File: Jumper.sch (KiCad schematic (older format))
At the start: 4 parts, among them J6 Conn_Coaxial, J7 Conn_Coaxial

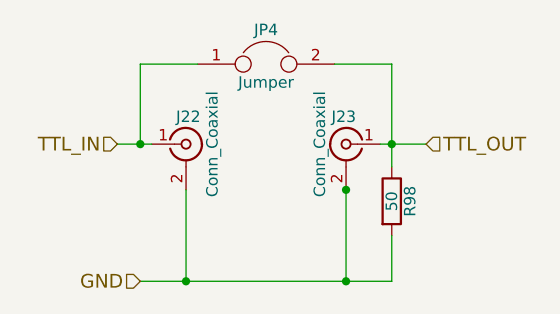
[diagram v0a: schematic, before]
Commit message: Version 1
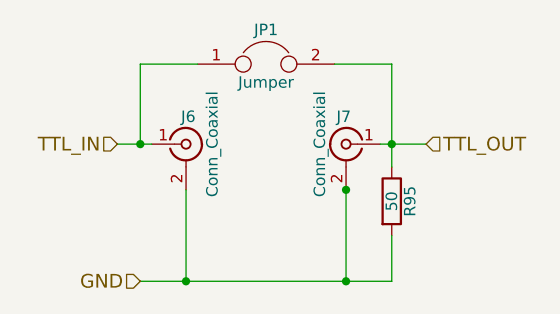
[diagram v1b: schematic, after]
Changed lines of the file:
@@
 AR Path="/59EF1109/59E237F4" Ref="J20"  Part="1"
 AR Path="/59EF2EEA/59E237F4" Ref="J22"  Part="1"
-F 0 "J22" H 4460 3920 50  0000 C CNN
+F 0 "J6" H 4460 3920 50  0000 C CNN
 F 1 "Conn_Coaxial" V 4565 3800 50  0000 C CNN
 F 2 "Connectors:LEMO_straight" H 4450 3800 50  0001 C CNN
@@
 AR Path="/59EF1109/59E23908" Ref="J21"  Part="1"
 AR Path="/59EF2EEA/59E23908" Ref="J23"  Part="1"
-F 0 "J23" H 5160 3920 50  0000 C CNN
+F 0 "J7" H 5160 3920 50  0000 C CNN
 F 1 "Conn_Coaxial" V 5265 3800 50  0000 C CNN
 F 2 "Connectors:LEMO_straight" H 5150 3800 50  0001 C CNN
@@
 AR Path="/59EF1109/59E23962" Ref="JP3"  Part="1"
 AR Path="/59EF2EEA/59E23962" Ref="JP4"  Part="1"
-F 0 "JP4" H 4800 3600 50  0000 C CNN
+F 0 "JP1" H 4800 3600 50  0000 C CNN
 F 1 "Jumper" H 4800 3370 50  0000 C CNN
 F 2 "Pin_Headers:Pin_Header_Straight_1x02_Pitch2.54mm" H 4800 3450 50  0001 C CNN
@@
 AR Path="/59EF1109/59F04D04" Ref="R97"  Part="1"
 AR Path="/59EF2EEA/59F04D04" Ref="R98"  Part="1"
-F 0 "R98" V 5430 4050 50  0000 C CNN
+F 0 "R95" V 5430 4050 50  0000 C CNN
 F 1 "50" V 5350 4050 50  0000 C CNN
 F 2 "Resistors_SMD:R_0805" V 5280 4050 50  0001 C CNN

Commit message: v1.1
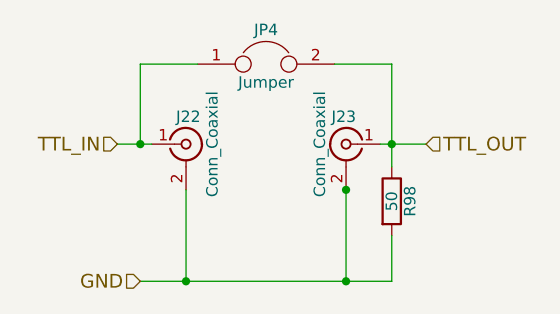
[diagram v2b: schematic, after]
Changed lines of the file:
@@
 AR Path="/59EF1109/59E237F4" Ref="J20"  Part="1"
 AR Path="/59EF2EEA/59E237F4" Ref="J22"  Part="1"
-F 0 "J6" H 4460 3920 50  0000 C CNN
+F 0 "J22" H 4460 3920 50  0000 C CNN
 F 1 "Conn_Coaxial" V 4565 3800 50  0000 C CNN
 F 2 "Connectors:LEMO_straight" H 4450 3800 50  0001 C CNN
@@
 AR Path="/59EF1109/59E23908" Ref="J21"  Part="1"
 AR Path="/59EF2EEA/59E23908" Ref="J23"  Part="1"
-F 0 "J7" H 5160 3920 50  0000 C CNN
+F 0 "J23" H 5160 3920 50  0000 C CNN
 F 1 "Conn_Coaxial" V 5265 3800 50  0000 C CNN
 F 2 "Connectors:LEMO_straight" H 5150 3800 50  0001 C CNN
@@
 AR Path="/59EF1109/59E23962" Ref="JP3"  Part="1"
 AR Path="/59EF2EEA/59E23962" Ref="JP4"  Part="1"
-F 0 "JP1" H 4800 3600 50  0000 C CNN
+F 0 "JP4" H 4800 3600 50  0000 C CNN
 F 1 "Jumper" H 4800 3370 50  0000 C CNN
 F 2 "Pin_Headers:Pin_Header_Straight_1x02_Pitch2.54mm" H 4800 3450 50  0001 C CNN
@@
 AR Path="/59EF1109/59F04D04" Ref="R97"  Part="1"
 AR Path="/59EF2EEA/59F04D04" Ref="R98"  Part="1"
-F 0 "R95" V 5430 4050 50  0000 C CNN
+F 0 "R98" V 5430 4050 50  0000 C CNN
 F 1 "50" V 5350 4050 50  0000 C CNN
 F 2 "Resistors_SMD:R_0805" V 5280 4050 50  0001 C CNN
